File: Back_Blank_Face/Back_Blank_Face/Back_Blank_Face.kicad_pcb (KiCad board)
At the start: 2 copper layers, 87 x 326.5 mm, 10 parts

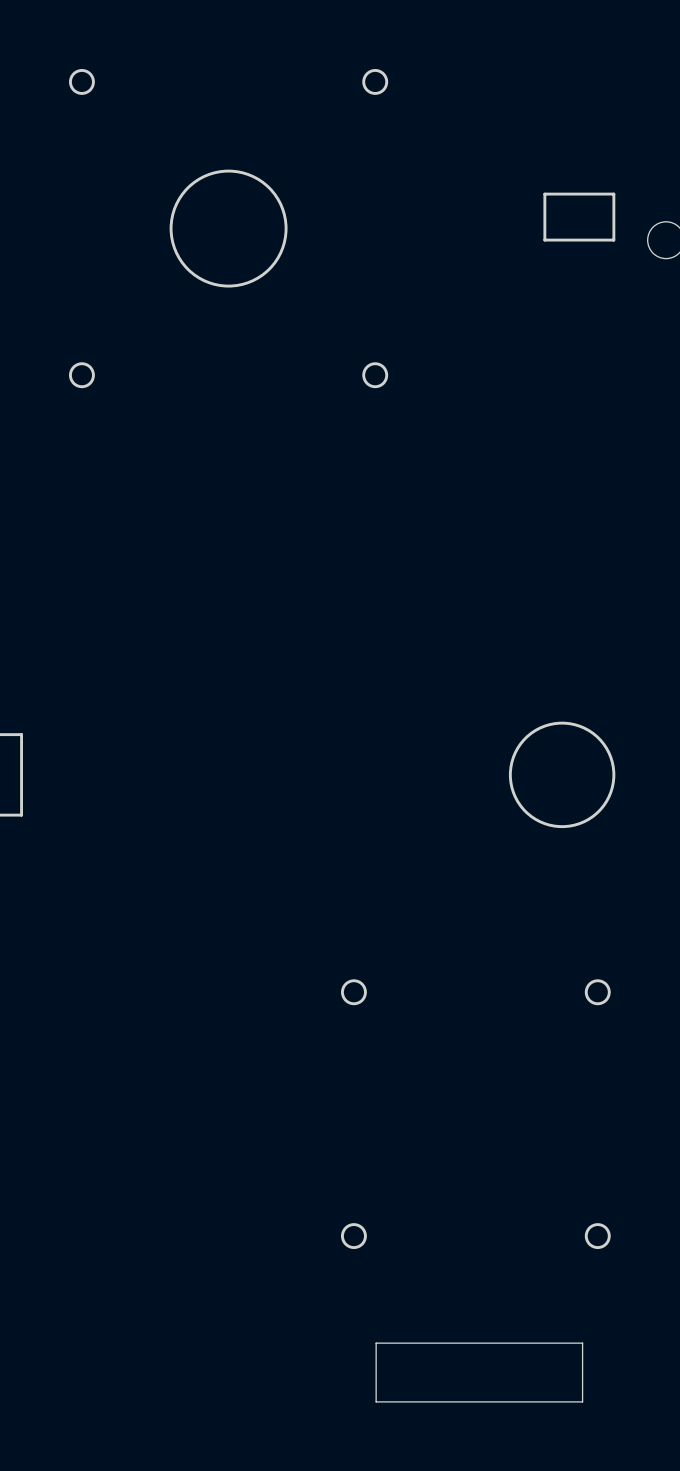
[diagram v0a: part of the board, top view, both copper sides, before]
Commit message: changed ALOT of things, got it to a point to send mech models,solar panel harness on BS need changed
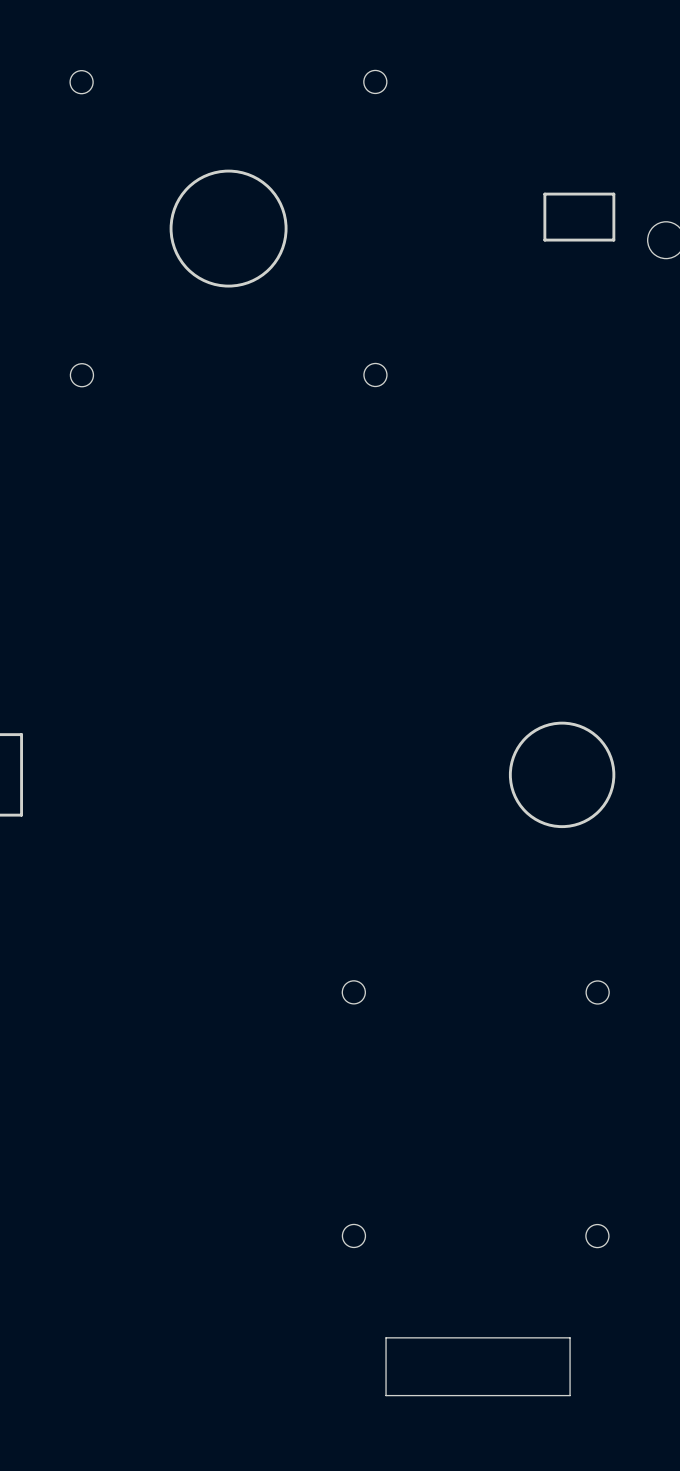
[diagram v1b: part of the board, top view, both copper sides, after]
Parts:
- added H15: MountingHole, Small_Mounting_Holes:2.0mm_Mounting_Hole, F.Cu at (147.1, -46.2)
- added H16: MountingHole, Small_Mounting_Holes:2.0mm_Mounting_Hole, F.Cu at (147.1, -20.7)
- added H17: MountingHole, Small_Mounting_Holes:2.0mm_Mounting_Hole, F.Cu at (121.6, -20.7)
- added H18: MountingHole, Small_Mounting_Holes:2.0mm_Mounting_Hole, F.Cu at (121.5, -46.2)
- added H19: MountingHole, Small_Mounting_Holes:2.0mm_Mounting_Hole, F.Cu at (166.4, 54.2)
- added H20: MountingHole, Small_Mounting_Holes:2.0mm_Mounting_Hole, F.Cu at (145.2, 54.2)
- added H21: MountingHole, Small_Mounting_Holes:2.0mm_Mounting_Hole, F.Cu at (166.4, 33.0)
- added H22: MountingHole, Small_Mounting_Holes:2.0mm_Mounting_Hole, F.Cu at (145.2, 33.0)
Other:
- outline, holes or cut-outs redrawn
